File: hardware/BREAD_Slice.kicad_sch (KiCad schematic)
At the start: 17 parts, among them J1 Conn_01x10_Female, U1 AP63205

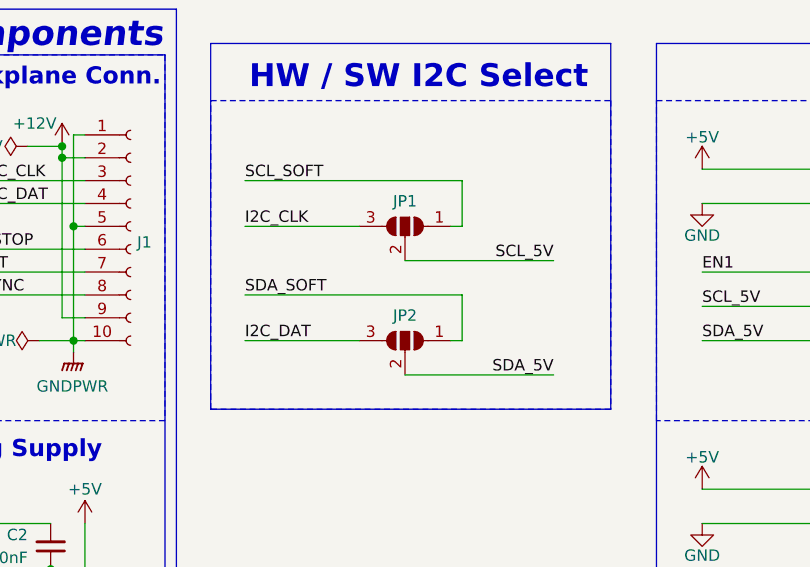
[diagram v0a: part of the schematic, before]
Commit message: chores: clean up warnings and part references
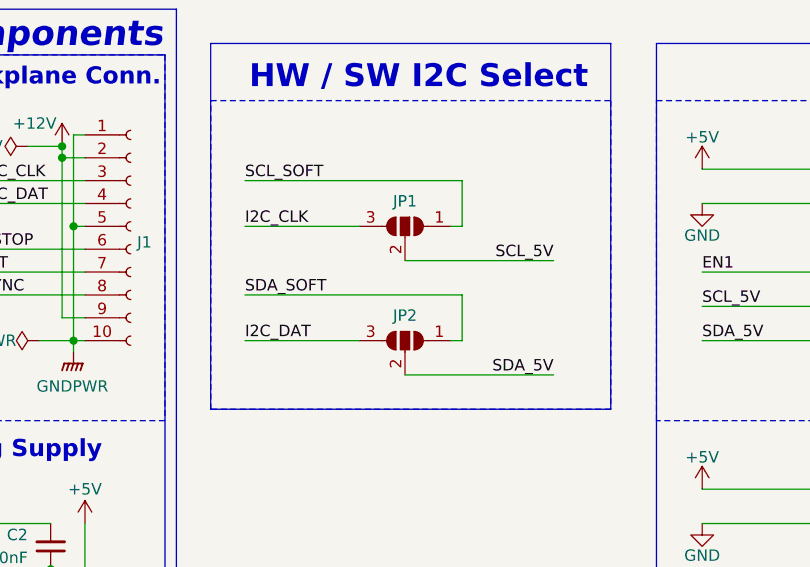
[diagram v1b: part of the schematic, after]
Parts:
- D1: footprint SparkFun-LED:WS2812-5050-4PIN -> KMLib_IC_SMD:WS2812-5050-4PIN; symbol SparkFun-LED:WS2812B_5050 -> KMLib_IC_Digital:WS2812B_5050_RGB_LED
- HS1: footprint kml-custom:Thermal Pad -> KMLib_Mounting:Thermal Pad
- J1: symbol Connector:Conn_01x10_Female -> Connector:Conn_01x10_Socket
- U1: footprint Package_TO_SOT_SMD:TSOT-23-6 -> KMLib_IC_SMD:SOIC_05WU-7_DIO; symbol SparkFun-DiscreteSemi:AP63205 -> KMLib_IC_Power:AP63205WU-7_Buck_Regulator
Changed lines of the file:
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@@
 	)
 	(symbol
-		(lib_id "Connector:Conn_01x10_Female")
+		(lib_id "Connector:Conn_01x10_Socket")
 		(at 60.96 36.83 0)
 		(unit 1)
@@
 			)
 		)
-		(property "Description" ""
+		(property "Description" "Generic connector, single row, 01x10, script generated"
 			(at 60.96 36.83 0)
 			(hide yes)
@@
 	)
 	(symbol
-		(lib_id "SparkFun-DiscreteSemi:AP63205")
+		(lib_id "KMLib_IC_Power:AP63205WU-7_Buck_Regulator")
 		(at 35.56 73.66 0)
 		(unit 1)
@@
 			)
 		)
-		(property "Footprint" "Package_TO_SOT_SMD:TSOT-23-6"
+		(property "Footprint" "KMLib_IC_SMD:SOIC_05WU-7_DIO"
 			(at 35.56 73.66 0)
 			(hide yes)
@@
 	)
 	(symbol
-		(lib_name "WS2812B_5050_1")
-		(lib_id "SparkFun-LED:WS2812B_5050")
+		(lib_id "KMLib_IC_Digital:WS2812B_5050_RGB_LED")
 		(at 30.48 40.64 0)
 		(unit 1)
@@
 			)
 		)
-		(property "Footprint" "SparkFun-LED:WS2812-5050-4PIN"
+		(property "Footprint" "KMLib_IC_SMD:WS2812-5050-4PIN"
 			(at 13.97 49.53 0)
 			(hide yes)
@@
 		)
 		(property "Datasheet" ""
-			(at 91.44 49.53 0)
+			(at 91.44 64.77 0)
 			(hide yes)
 			(show_name no)
@@
 		)
 		(property "Description" "Solder Jumper, 3-pole, open"
-			(at 91.44 49.53 0)
+			(at 91.44 62.23 0)
 			(hide yes)
 			(show_name no)
@@
 			)
 		)
-		(property "Footprint" "kml-custom:Thermal Pad"
+		(property "Footprint" "KMLib_Mounting:Thermal Pad"
 			(at 35.8648 97.79 0)
 			(hide yes)
@@
 		)
 		(property "Datasheet" ""
-			(at 91.44 36.83 0)
+			(at 91.44 52.07 0)
 			(hide yes)
 			(show_name no)
@@
 		)
 		(property "Description" "Solder Jumper, 3-pole, open"
-			(at 91.44 36.83 0)
-			(hide yes)
-			(show_name no)
+			(at 91.44 49.53 0)
+			(hide yes)
+			(show_name no)

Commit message: fix(hw): re-point stale library nicknames
These parts exist in KiCad-Master-Lib; the boards referenced libraries that no
longer exist (kml-custom, KML-Custom, and SparkFun libraries that never
contained the part) or names the library has since changed.

KiCad embeds footprint geometry in the .kicad_pcb, so the boards rendered and
fabricated correctly and the rot stayed invisible -- it only surfaces on
update-from-library, or when a generator tries to resolve a nickname.

Nickname/name only. No geometry is changed:

  KMLib_Mounting:Thermal Pad -> KMLib_Mounting:Thermal_Pad
  SparkFun-LED:WS2812-5050-4PIN -> KMLib_IC_SMD:WS2812-5050-4PIN
  kml-custom:Atlas_OEM -> KMLib_Boards_Modules:Atlas_OEM
  kml-custom:FAST-Logo-XXXLarge -> KMLib_Aesthetic:FAST-Logo-XXXLarge
  kml-custom:RS_20_ADI-L -> KMLib_IC_SMD:RS_20_ADI-L
  kml-custom:Thermal Pad -> KMLib_Mounting:Thermal_Pad

Only references that failed to resolve were touched. Generic parts (<=4 pins)
and KiCad *-rescue libraries are deliberately excluded: fingerprint matching
cannot distinguish a 2-pin resistor from a 2-pin capacitor, so those are being
done by hand.
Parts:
- HS1: footprint KMLib_Mounting:Thermal Pad -> KMLib_Mounting:Thermal_Pad
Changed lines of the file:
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@@
 			)
 		)
-		(property "Footprint" "KMLib_Mounting:Thermal Pad"
+		(property "Footprint" "KMLib_Mounting:Thermal_Pad"
 			(at 35.8648 97.79 0)
 			(hide yes)
